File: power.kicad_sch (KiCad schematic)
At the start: 13 parts, among them J1 USB_B_Micro, U2 S2B-PH-K-S-GW, U3 AP2112K-3.3TRG1, U4 MCP73831T-2ACI/OT, U6 MSK-12C02_SMD_SPDT_SWITCH

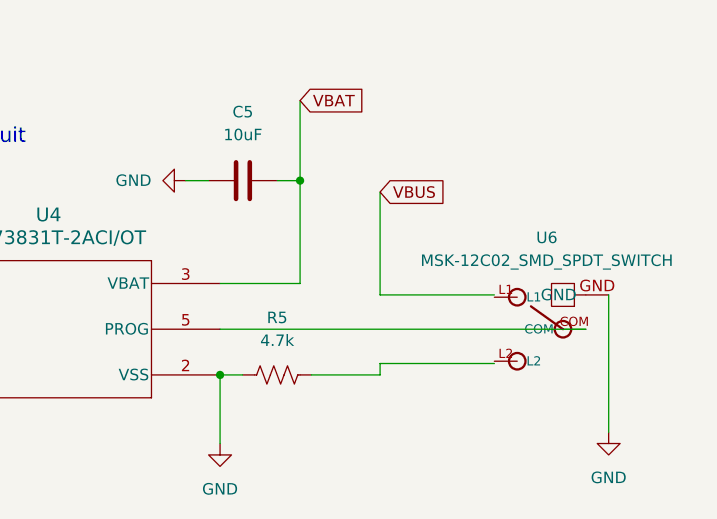
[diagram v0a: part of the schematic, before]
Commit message: PCB Smol Time
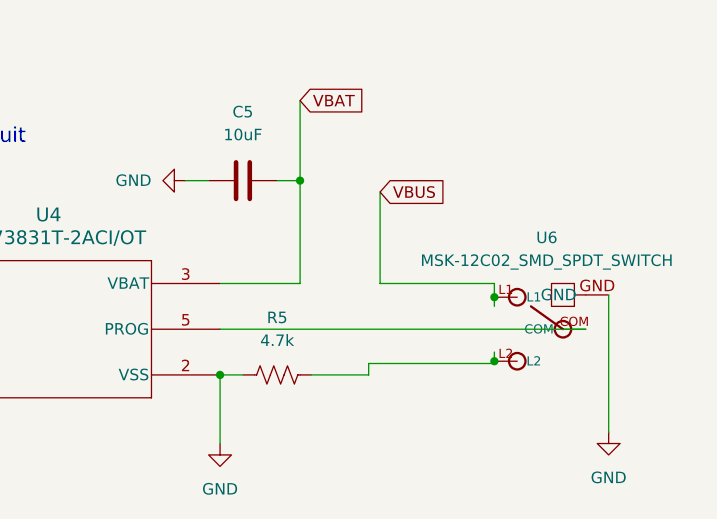
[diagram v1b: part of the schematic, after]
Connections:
- net VBUS: now also U6.L1
- net at U6.L2: now also R5.2
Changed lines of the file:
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@@
+	)
+	(junction
+		(at 252.73 64.516)
+		(diameter 0)
+		(color 0 0 0 0)
 	)
 	(junction
@@
 	)
 	(junction
+		(at 252.73 57.404)
+		(diameter 0)
+		(color 0 0 0 0)
+	)
+	(junction
 		(at 91.44 54.61)
 		(diameter 0)
@@
 	(wire
 		(pts
+			(xy 252.73 55.88) (xy 252.73 57.404)
+		)
+		(stroke
+			(width 0)
+			(type default)
+		)
+	)
+	(wire
+		(pts
 			(xy 33.02 54.61) (xy 29.21 54.61)
 		)
@@
 	(wire
 		(pts
-			(xy 240.03 66.04) (xy 232.41 66.04)
-		)
-		(stroke
-			(width 0)
-			(type default)
-		)
-	)
-	(wire
-		(pts
-			(xy 240.03 64.77) (xy 240.03 66.04)
+			(xy 238.76 66.04) (xy 232.41 66.04)
+		)
+		(stroke
+			(width 0)
+			(type default)
+		)
+	)
+	(wire
+		(pts
+			(xy 238.76 64.77) (xy 238.76 66.04)
 		)
 		(stroke
@@
 	(wire
 		(pts
-			(xy 240.03 57.15) (xy 252.73 57.15)
+			(xy 240.03 55.88) (xy 252.73 55.88)
+		)
+		(stroke
+			(width 0)
+			(type default)
+		)
+	)
+	(wire
+		(pts
+			(xy 252.73 57.404) (xy 252.73 58.42)
 		)
 		(stroke
@@
 	(wire
 		(pts
+			(xy 252.73 63.5) (xy 252.73 64.516)
+		)
+		(stroke
+			(width 0)
+			(type default)
+		)
+	)
+	(wire
+		(pts
 			(xy 91.44 64.77) (xy 91.44 69.85)
 		)
@@
 	(wire
 		(pts
-			(xy 240.03 64.77) (xy 252.73 64.77)
+			(xy 238.76 64.77) (xy 252.73 64.77)
 		)
 		(stroke
@@
 	(wire
 		(pts
-			(xy 240.03 45.72) (xy 240.03 57.15)
+			(xy 240.03 45.72) (xy 240.03 55.88)
 		)
 		(stroke
@@
 		)
 		(stroke
+			(width 0)
+			(type default)
+		)
+	)
+	(wire
+		(pts
+			(xy 252.73 64.516) (xy 252.73 64.77)
+		)
+		(stroke

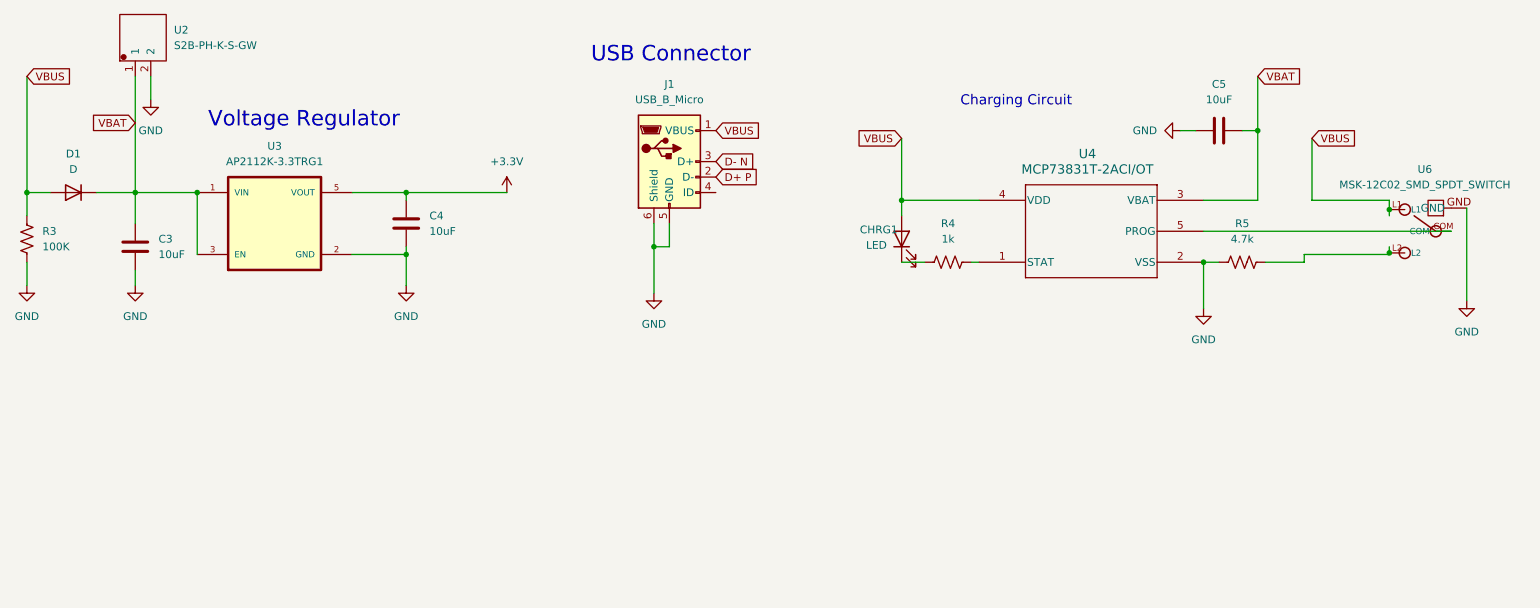
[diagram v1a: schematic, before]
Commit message: update power circuit
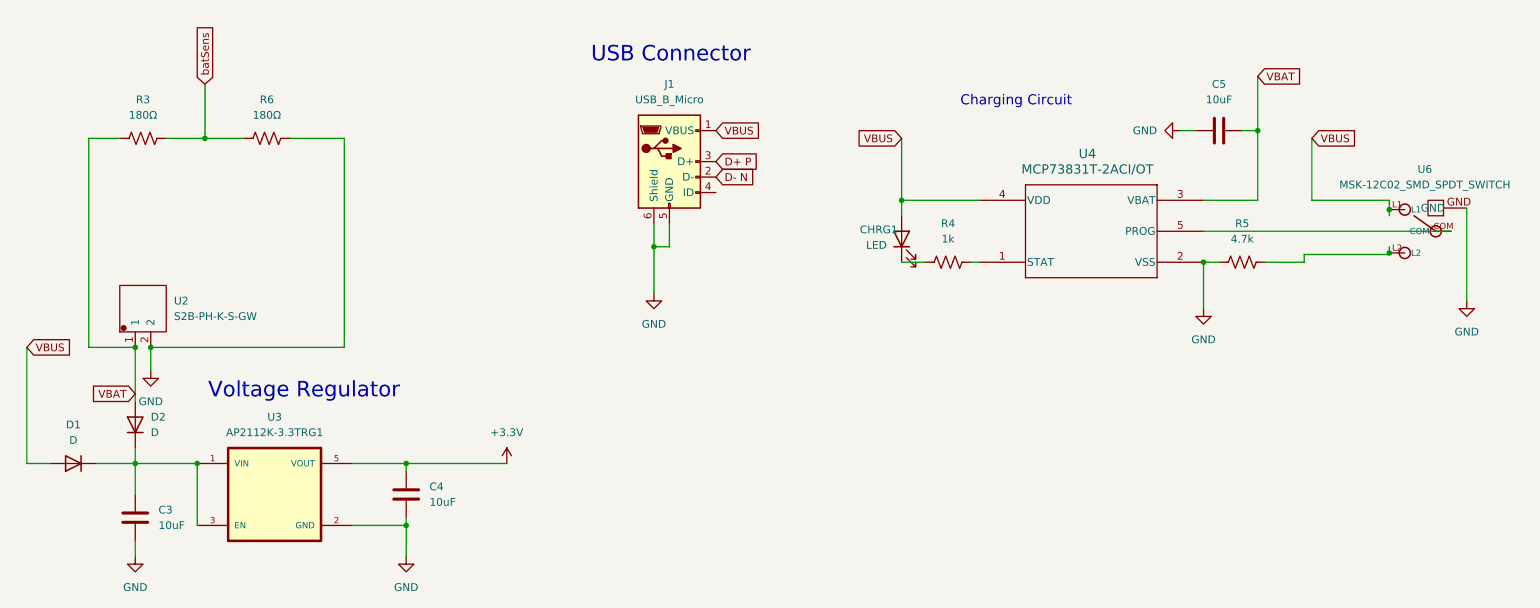
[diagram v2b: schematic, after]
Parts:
- added D2: D, Diode_SMD:D_0603_1608Metric, symbol uSlime:D
- added R6: 180Ω, Resistor_SMD:R_0402_1005Metric, symbol uSlime:R_US
- R3: value 100K -> 180Ω
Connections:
- net D+ P: now also J1.3 (D+); no longer J1.2 (D-)
- net D- N: now also J1.2 (D-); no longer J1.3 (D+)
- net GND: now also R6.2; no longer R3.2
- net VBAT: now also R3.1, D2.2 (A); no longer C3.1, D1.1 (K), U3.1 (VIN), U3.3 (EN)
- net VBUS: no longer R3.1
- new net: C3.1, D1.1 (K), D2.1 (K), U3.1 (VIN), U3.3 (EN)
- new net batSens: R3.2, R6.1
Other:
- moved on the sheet: C3, C4, D1, U2, U3
